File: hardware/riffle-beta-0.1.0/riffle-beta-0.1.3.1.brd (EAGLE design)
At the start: 104.8 x 18 mm, 46 parts, among them IC1 ATMEGA328P, IC3 CH340G, IC4 MCP1700-33, IC5 24AA128SN, IC6 MCP1700-33, J1 AYZ0202, U1 MCP73831T-2ACI/OT, X2 12MHz, X3 16 MHz

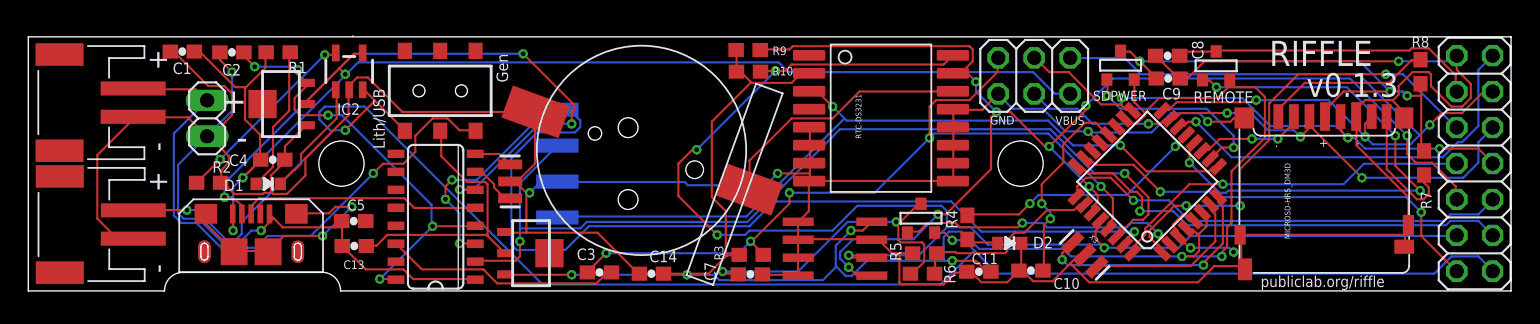
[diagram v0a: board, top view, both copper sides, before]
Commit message: update
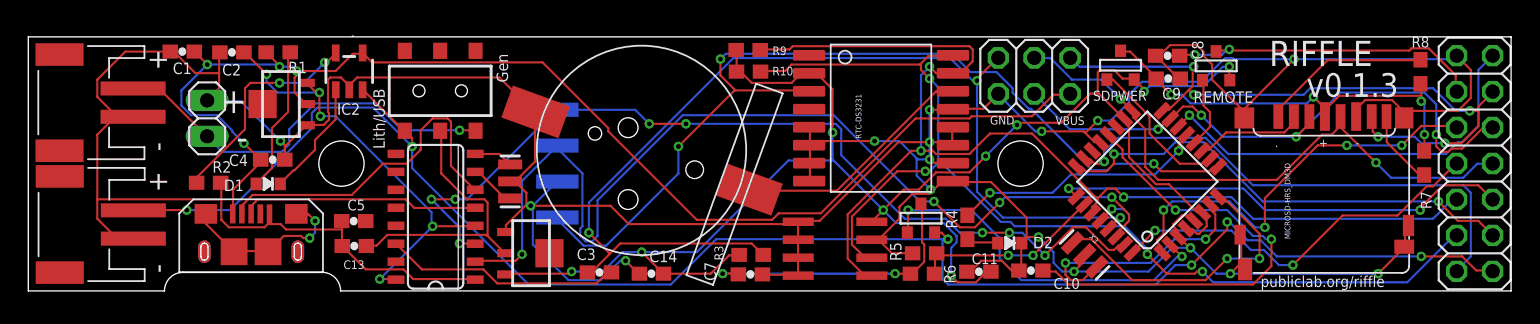
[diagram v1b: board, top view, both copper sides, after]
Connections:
- net GND: now also JP1.2; no longer JP1.1
- net VGEN: now also JP1.1; no longer JP1.2
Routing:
- net D8: track 38.7 -> 5.11 mm, vias 4 -> 0
- net D-: track 45.4 -> 24.4 mm, vias 4 -> 0
- net AREF: track 14.2 -> 33.9 mm
- net SCL: track 97.0 -> 78.4 mm
- net RESET: track 56.2 -> 72.3 mm, vias 5 -> 3
- net TXD: track 77.7 -> 63.6 mm, vias 4 -> 8
- net VGEN: track 41.8 -> 28.9 mm
- net D5/RTC: track 54.6 -> 66.5 mm, vias 2 -> 3
- net GND: track 315.4 -> 326.1 mm, vias 9 -> 16
- net VCC: track 122.8 -> 114.5 mm, vias 6 -> 9
- net SDA: track 89.9 -> 81.6 mm, vias 8 -> 3
- net MISO: track 55.1 -> 47.0 mm, vias 3 -> 5
- net D4: track 20.1 -> 25.7 mm
- net A0: track 30.6 -> 36.2 mm, vias 2 -> 1
- net N$2: track 11.9 -> 17.1 mm, vias 0 -> 2
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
